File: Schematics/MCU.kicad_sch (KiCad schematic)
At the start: 4 parts, among them U1 ATmega64A-A, Y1 16MHz

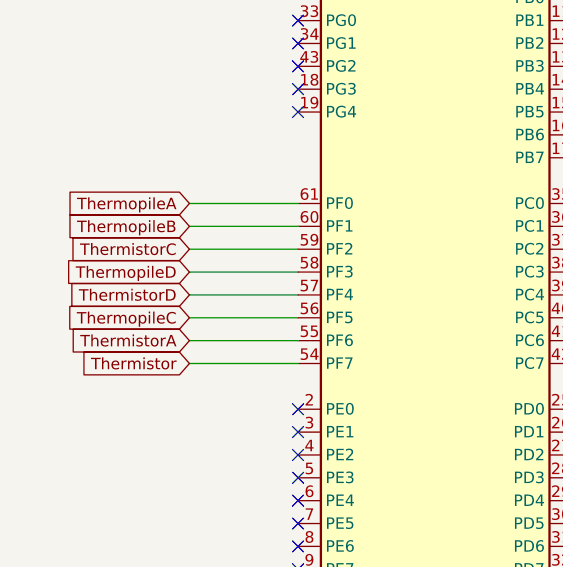
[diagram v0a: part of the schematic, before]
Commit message: PCB
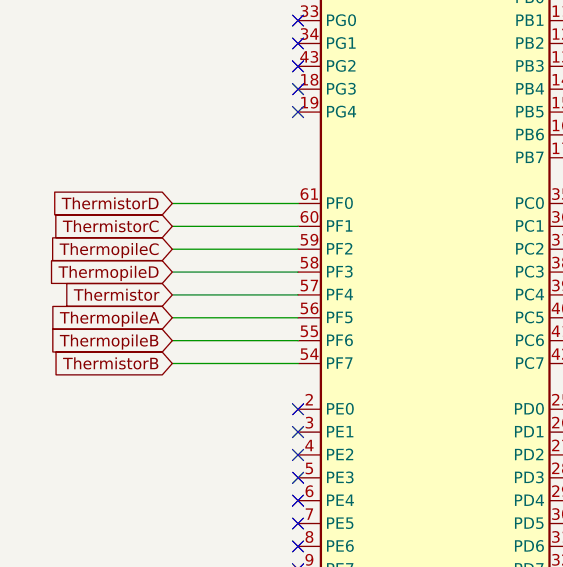
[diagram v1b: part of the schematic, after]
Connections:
- net ThermistorA is gone; now on net ThermopileB: U1.55 (PF6)
- net Thermistor: now also U1.57 (PF4); no longer U1.54 (PF7)
- net ThermistorC: now also U1.60 (PF1); no longer U1.59 (PF2)
- net ThermistorD: now also U1.61 (PF0); no longer U1.57 (PF4)
- net ThermopileA: now also U1.56 (PF5); no longer U1.61 (PF0)
- net ThermopileB: no longer U1.60 (PF1)
- net ThermopileC: now also U1.59 (PF2); no longer U1.56 (PF5)
- new net ThermistorB: U1.54 (PF7)
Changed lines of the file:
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@@
   (no_connect (at 162.56 68.58))
   (no_connect (at 162.56 71.12))
+  (wire (pts (xy 118.11 109.22) (xy 132.08 109.22))
+    (stroke (width 0) (type default) (color 0 0 0 0))
+  )
   (wire (pts (xy 162.56 88.9) (xy 174.625 88.9))
     (stroke (width 0) (type default) (color 0 0 0 0))
   )
+  (wire (pts (xy 118.11 106.68) (xy 132.08 106.68))
+    (stroke (width 0) (type default) (color 0 0 0 0))
+  )
   (wire (pts (xy 107.95 71.12) (xy 107.95 76.2))
     (stroke (width 0) (type default) (color 0 0 0 0))
@@
     (stroke (width 0) (type default) (color 0 0 0 0))
   )
-  (wire (pts (xy 120.015 109.22) (xy 132.08 109.22))
-    (stroke (width 0) (type default) (color 0 0 0 0))
-  )
   (wire (pts (xy 127 81.28) (xy 132.08 81.28))
     (stroke (width 0) (type default) (color 0 0 0 0))
   )
-  (wire (pts (xy 120.015 114.3) (xy 132.08 114.3))
-    (stroke (width 0) (type default) (color 0 0 0 0))
-  )
   (wire (pts (xy 149.86 45.72) (xy 147.32 45.72))
     (stroke (width 0) (type default) (color 0 0 0 0))
   )
+  (wire (pts (xy 118.11 111.76) (xy 132.08 111.76))
+    (stroke (width 0) (type default) (color 0 0 0 0))
+  )
   (wire (pts (xy 125.73 71.12) (xy 132.08 71.12))
     (stroke (width 0) (type default) (color 0 0 0 0))
@@
     (stroke (width 0) (type default) (color 0 0 0 0))
   )
-  (wire (pts (xy 120.015 111.76) (xy 132.08 111.76))
-    (stroke (width 0) (type default) (color 0 0 0 0))
-  )
-  (wire (pts (xy 120.015 119.38) (xy 132.08 119.38))
-    (stroke (width 0) (type default) (color 0 0 0 0))
-  )
   (wire (pts (xy 149.86 53.34) (xy 149.86 45.72))
     (stroke (width 0) (type default) (color 0 0 0 0))
   )
-  (wire (pts (xy 120.015 124.46) (xy 132.08 124.46))
-    (stroke (width 0) (type default) (color 0 0 0 0))
-  )
   (wire (pts (xy 162.56 91.44) (xy 174.625 91.44))
     (stroke (width 0) (type default) (color 0 0 0 0))
@@
     (stroke (width 0) (type default) (color 0 0 0 0))
   )
-  (wire (pts (xy 120.015 121.92) (xy 132.08 121.92))
-    (stroke (width 0) (type default) (color 0 0 0 0))
-  )
   (wire (pts (xy 162.56 66.04) (xy 175.26 66.04))
     (stroke (width 0) (type default) (color 0 0 0 0))
@@
     (stroke (width 0) (type default) (color 0 0 0 0))
   )
+  (wire (pts (xy 118.11 119.38) (xy 132.08 119.38))
+    (stroke (width 0) (type default) (color 0 0 0 0))
+  )
   (wire (pts (xy 119.38 66.04) (xy 125.73 66.04))
     (stroke (width 0) (type default) (color 0 0 0 0))
   )
-  (wire (pts (xy 120.015 116.84) (xy 132.08 116.84))
+  (wire (pts (xy 118.11 114.3) (xy 132.08 114.3))
+    (stroke (width 0) (type default) (color 0 0 0 0))
+  )
+  (wire (pts (xy 118.11 116.84) (xy 132.08 116.84))
     (stroke (width 0) (type default) (color 0 0 0 0))
   )
@@
     (stroke (width 0) (type default) (color 0 0 0 0))
   )
-  (wire (pts (xy 120.015 106.68) (xy 132.08 106.68))
+  (wire (pts (xy 118.11 124.46) (xy 132.08 124.46))
+    (stroke (width 0) (type default) (color 0 0 0 0))
+  )
+  (wire (pts (xy 118.11 121.92) (xy 132.08 121.92))
     (stroke (width 0) (type default) (color 0 0 0 0))
   )
@@
     (stroke (width 0) (type default) (color 0 0 0 0))
   )
-  (global_label "ThermistorD" (shape input) (at 120.015 116.84 180) (fields_autoplaced)
-    (effects (font (size 1.27 1.27)) (justify right))
-    (property "Intersheet References" "${INTERSHEET_REFS}" (id 0) (at 106.3533 116.9194 0)
+  (global_label "ThermistorD" (shape input) (at 118.11 106.68 180) (fields_autoplaced)
+    (effects (font (size 1.27 1.27)) (justify right))
+    (property "Intersheet References" "${INTERSHEET_REFS}" (id 0) (at 104.4483 106.7594 0)
       (effects (font (size 1.27 1.27)) (justify right) hide)
     )
@@
     )
   )
-  (global_label "ThermopileC" (shape input) (at 120.015 119.38 180) (fields_autoplaced)
-    (effects (font (size 1.27 1.27)) (justify right))
-    (property "Intersheet References" "${INTERSHEET_REFS}" (id 0) (at 105.9905 119.4594 0)
+  (global_label "ThermopileC" (shape input) (at 118.11 111.76 180) (fields_autoplaced)
+    (effects (font (size 1.27 1.27)) (justify right))
+    (property "Intersheet References" "${INTERSHEET_REFS}" (id 0) (at 104.0855 111.8394 0)
       (effects (font (size 1.27 1.27)) (justify right) hide)
     )
@@
     )
   )
-  (global_label "ThermopileA" (shape input) (at 120.015 106.68 180) (fields_autoplaced)
-    (effects (font (size 1.27 1.27)) (justify right))
-    (property "Intersheet References" "${INTERSHEET_REFS}" (id 0) (at 106.1719 106.7594 0)
-      (effects (font (size 1.27 1.27)) (justify right) hide)
-    )
-  )
   (global_label "ServoPWM" (shape input) (at 174.625 60.96 0) (fields_autoplaced)
     (effects (font (size 1.27 1.27)) (justify left))
@@
     )
   )
+  (global_label "ThermopileB" (shape input) (at 118.11 121.92 180) (fields_autoplaced)
+    (effects (font (size 1.27 1.27)) (justify right))
+    (property "Intersheet References" "${INTERSHEET_REFS}" (id 0) (at 104.0855 121.8406 0)
+      (effects (font (size 1.27 1.27)) (justify right) hide)
+    )
+  )
   (global_label "~{RESET}" (shape input) (at 120.015 60.96 180) (fields_autoplaced)
     (effects (font (size 1.27 1.27)) (justify right))
@@
     )
   )
-  (global_label "ThermistorC" (shape input) (at 120.015 111.76 180) (fields_autoplaced)
-    (effects (font (size 1.27 1.27)) (justify right))
-    (property "Intersheet References" "${INTERSHEET_REFS}" (id 0) (at 106.3533 111.6806 0)
-      (effects (font (size 1.27 1.27)) (justify right) hide)
-    )
-  )
-  (global_label "ThermopileD" (shape input) (at 120.015 114.3 180) (fields_autoplaced)
-    (effects (font (size 1.27 1.27)) (justify right))
-    (property "Intersheet References" "${INTERSHEET_REFS}" (id 0) (at 105.9905 114.2206 0)
-      (effects (font (size 1.27 1.27)) (justify right) hide)
-    )
-  )
-  (global_label "ThermistorA" (shape input) (at 120.015 121.92 180) (fields_autoplaced)
-    (effects (font (size 1.27 1.27)) (justify right))
-    (property "Intersheet References" "${INTERSHEET_REFS}" (id 0) (at 106.5348 121.8406 0)
+  (global_label "ThermistorC" (shape input) (at 118.11 109.22 180) (fields_autoplaced)
+    (effects (font (size 1.27 1.27)) (justify right))
+    (property "Intersheet References" "${INTERSHEET_REFS}" (id 0) (at 104.4483 109.1406 0)
+      (effects (font (size 1.27 1.27)) (justify right) hide)
+    )
+  )
+  (global_label "ThermopileD" (shape input) (at 118.11 114.3 180) (fields_autoplaced)
+    (effects (font (size 1.27 1.27)) (justify right))
+    (property "Intersheet References" "${INTERSHEET_REFS}" (id 0) (at 104.0855 114.2206 0)
+      (effects (font (size 1.27 1.27)) (justify right) hide)
+    )
+  )
+  (global_label "ThermistorB" (shape input) (at 118.11 124.46 180) (fields_autoplaced)
+    (effects (font (size 1.27 1.27)) (justify right))
+    (property "Intersheet References" "${INTERSHEET_REFS}" (id 0) (at 104.4483 124.3806 0)
       (effects (font (size 1.27 1.27)) (justify right) hide)
     )
@@
     )
   )
+  (global_label "ThermopileA" (shape input) (at 118.11 119.38 180) (fields_autoplaced)
+    (effects (font (size 1.27 1.27)) (justify right))
+    (property "Intersheet References" "${INTERSHEET_REFS}" (id 0) (at 104.2669 119.4594 0)
+      (effects (font (size 1.27 1.27)) (justify right) hide)
+    )
+  )
   (global_label "SCK" (shape input) (at 174.625 86.36 0) (fields_autoplaced)
     (effects (font (size 1.27 1.27)) (justify left))
@@
     )
   )
-  (global_label "ThermopileB" (shape input) (at 120.015 109.22 180) (fields_autoplaced)
-    (effects (font (size 1.27 1.27)) (justify right))
-    (property "Intersheet References" "${INTERSHEET_REFS}" (id 0) (at 105.9905 109.1406 0)
-      (effects (font (size 1.27 1.27)) (justify right) hide)
-    )
-  )
   (global_label "MOSI" (shape input) (at 174.625 88.9 0) (fields_autoplaced)
     (effects (font (size 1.27 1.27)) (justify left))
@@
     )
   )
-  (global_label "Thermistor" (shape input) (at 120.015 124.46 180) (fields_autoplaced)
-    (effects (font (size 1.27 1.27)) (justify right))
-    (property "Intersheet References" "${INTERSHEET_REFS}" (id 0) (at 107.6233 124.3806 0)
-      (effects (font (size 1.27 1.27)) (justify right) hide)
-    )
+  (global_label "Thermistor" (shape input) (at 118.11 116.84 180) (fields_autoplaced)
+    (effects (font (size 1.27 1.27)) (justify right))
+    (property "Intersheet References" "${INTERSHEET_REFS}" (id 0) (at 105.7183 116.7606 0)
+      (effects (font (size 1.27 1.27)) (justify right) hide)
+    )

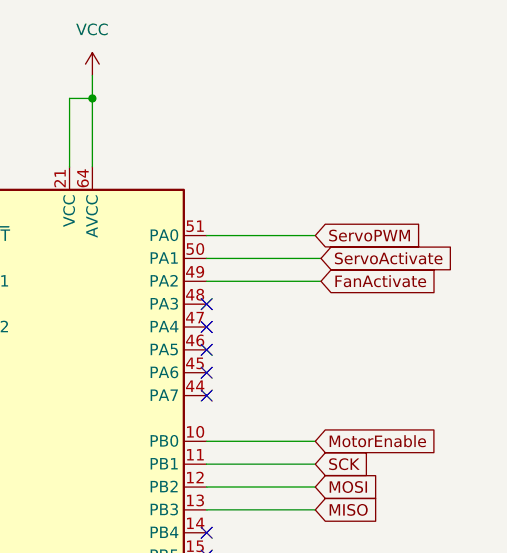
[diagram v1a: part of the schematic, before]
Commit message: PCB
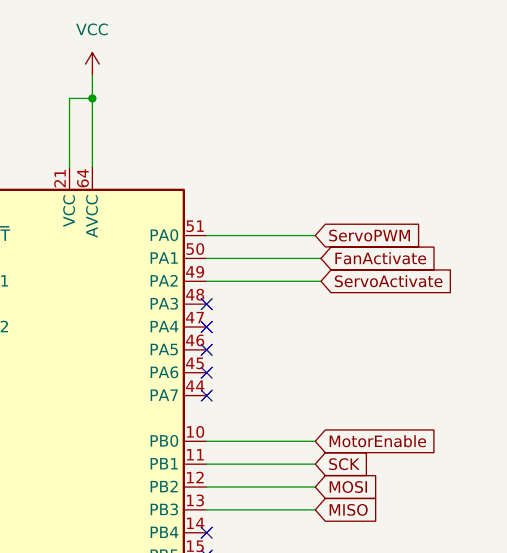
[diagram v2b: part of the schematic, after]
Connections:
- net FanActivate: now also U1.50 (PA1); no longer U1.49 (PA2)
- net ServoActivate: now also U1.49 (PA2); no longer U1.50 (PA1)
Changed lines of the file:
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@@
     )
   )
-  (global_label "ServoActivate" (shape input) (at 175.26 63.5 0) (fields_autoplaced)
+  (global_label "ServoActivate" (shape input) (at 175.26 66.04 0) (fields_autoplaced)
     (effects (font (size 1.27 1.27)) (justify left))
-    (property "Intersheet References" "${INTERSHEET_REFS}" (id 0) (at 190.3126 63.4206 0)
+    (property "Intersheet References" "${INTERSHEET_REFS}" (id 0) (at 190.3126 65.9606 0)
       (effects (font (size 1.27 1.27)) (justify left) hide)
     )
@@
     )
   )
-  (global_label "FanActivate" (shape input) (at 175.26 66.04 0) (fields_autoplaced)
+  (global_label "FanActivate" (shape input) (at 175.26 63.5 0) (fields_autoplaced)
     (effects (font (size 1.27 1.27)) (justify left))
-    (property "Intersheet References" "${INTERSHEET_REFS}" (id 0) (at 188.4983 65.9606 0)
+    (property "Intersheet References" "${INTERSHEET_REFS}" (id 0) (at 188.4983 63.4206 0)
       (effects (font (size 1.27 1.27)) (justify left) hide)
     )
